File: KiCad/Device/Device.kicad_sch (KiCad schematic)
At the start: 25 parts, among them IC1 ATTINY167-XUR, J1 Mikrofon, J2 Lysføler, J3 Optisk sensor, J4 Fugtføler, J5 VCC, J6 ESP8266(wifi), SW1 Reset, SW2 Button01, SW3 SW_DIP_x01, Y1 Crystal

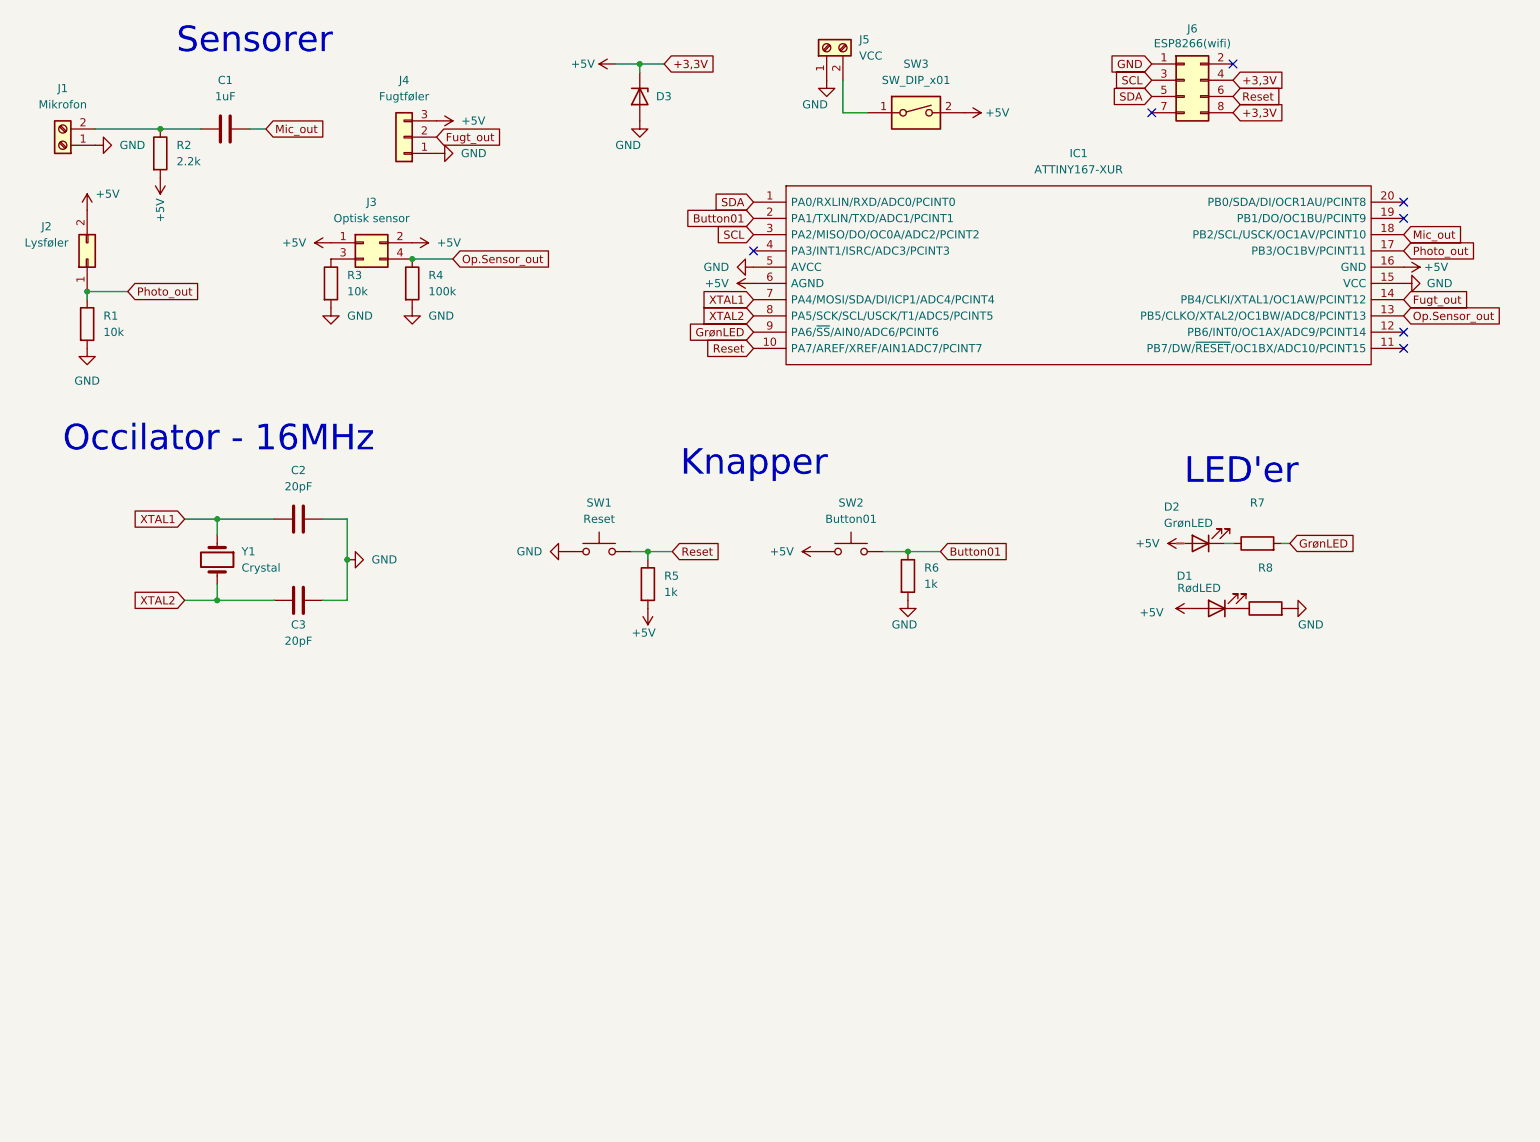
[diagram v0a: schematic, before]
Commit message: Minor fixes
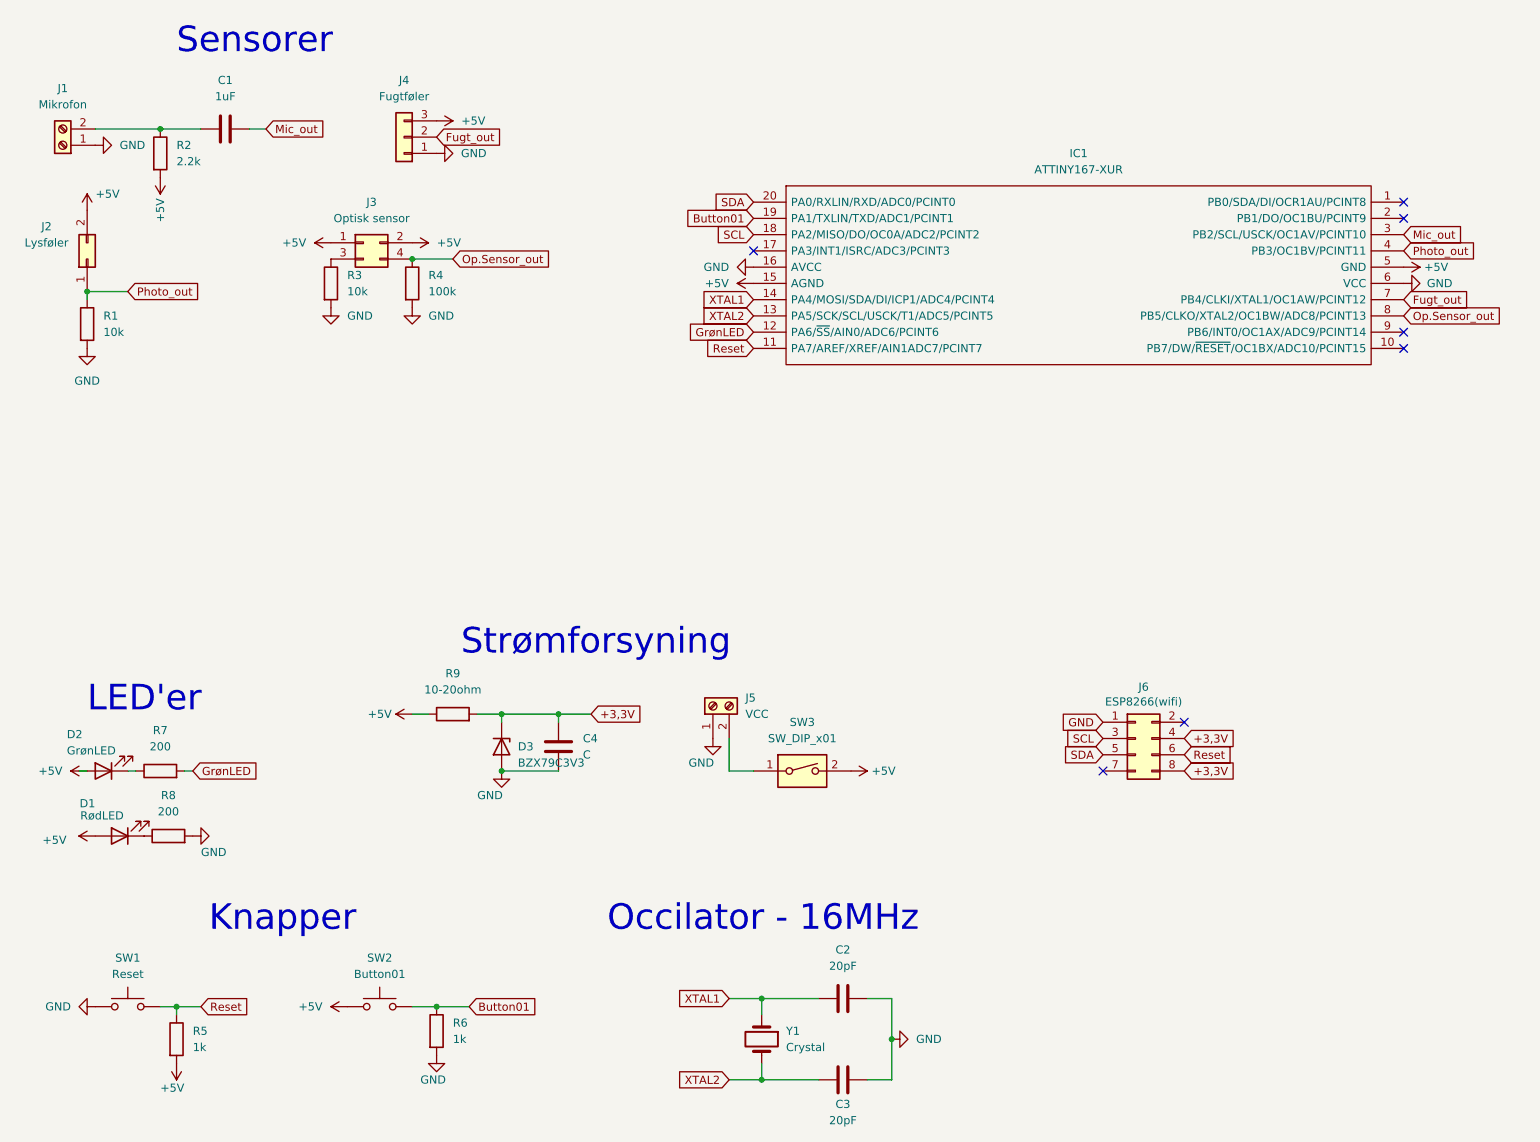
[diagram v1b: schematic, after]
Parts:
- added C4: C, symbol Device:C
- added R9: 10-20ohm, Resistor_THT:R_Axial_DIN0309_L9.0mm_D3.2mm_P12.70mm_Horizontal, symbol Device:R
- D3: value (none) -> BZX79C3V3; footprint (none) -> Diode_SMD:D_MELF_Handsoldering
- IC1: footprint (none) -> Package_DIP:DIP-20_W7.62mm_Socket
- R7, R8: value (none) -> 200
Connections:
- net +5V: now also IC1.15 (AGND), IC1.5 (GND), R9.1; no longer D3.1 (K), IC1.16 (GND), IC1.6 (AGND), J6.4 (Pin_4), J6.8 (Pin_8)
- net Button01: now also IC1.19 (PA1/TXLIN/TXD/ADC1/PCINT1); no longer IC1.2 (PA1/TXLIN/TXD/ADC1/PCINT1)
- net Fugt_out: now also IC1.7 (PB4/CLKI/XTAL1/OC1AW/PCINT12); no longer IC1.14 (PB4/CLKI/XTAL1/OC1AW/PCINT12)
- net GND: now also IC1.16 (AVCC), IC1.6 (VCC), C4.2; no longer IC1.15 (VCC), IC1.5 (AVCC)
- net GrønLED: now also IC1.12 (PA6/~{SS}/AIN0/ADC6/PCINT6); no longer IC1.9 (PA6/~{SS}/AIN0/ADC6/PCINT6)
- net Mic_out: now also IC1.3 (PB2/SCL/USCK/OC1AV/PCINT10); no longer IC1.18 (PB2/SCL/USCK/OC1AV/PCINT10)
- net Op.Sensor_out: now also IC1.8 (PB5/CLKO/XTAL2/OC1BW/ADC8/PCINT13); no longer IC1.13 (PB5/CLKO/XTAL2/OC1BW/ADC8/PCINT13)
- net Photo_out: now also IC1.4 (PB3/OC1BV/PCINT11); no longer IC1.17 (PB3/OC1BV/PCINT11)
- net Reset: now also IC1.11 (PA7/AREF/XREF/AIN1ADC7/PCINT7); no longer IC1.10 (PA7/AREF/XREF/AIN1ADC7/PCINT7)
- net SCL: now also IC1.18 (PA2/MISO/DO/OC0A/ADC2/PCINT2); no longer IC1.3 (PA2/MISO/DO/OC0A/ADC2/PCINT2)
- net SDA: now also IC1.20 (PA0/RXLIN/RXD/ADC0/PCINT0); no longer IC1.1 (PA0/RXLIN/RXD/ADC0/PCINT0)
- net XTAL1: now also IC1.14 (PA4/MOSI/SDA/DI/ICP1/ADC4/PCINT4); no longer IC1.7 (PA4/MOSI/SDA/DI/ICP1/ADC4/PCINT4)
- net XTAL2: now also IC1.13 (PA5/SCK/SCL/USCK/T1/ADC5/PCINT5); no longer IC1.8 (PA5/SCK/SCL/USCK/T1/ADC5/PCINT5)
- new net +3,3V: C4.1, D3.1 (K), J6.4 (Pin_4), J6.8 (Pin_8), R9.2
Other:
- note added: "Strømforsyning"
- moved on the sheet: C2, C3, D1, D2, D3, J5, J6, R5, R6, R7, R8, SW1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

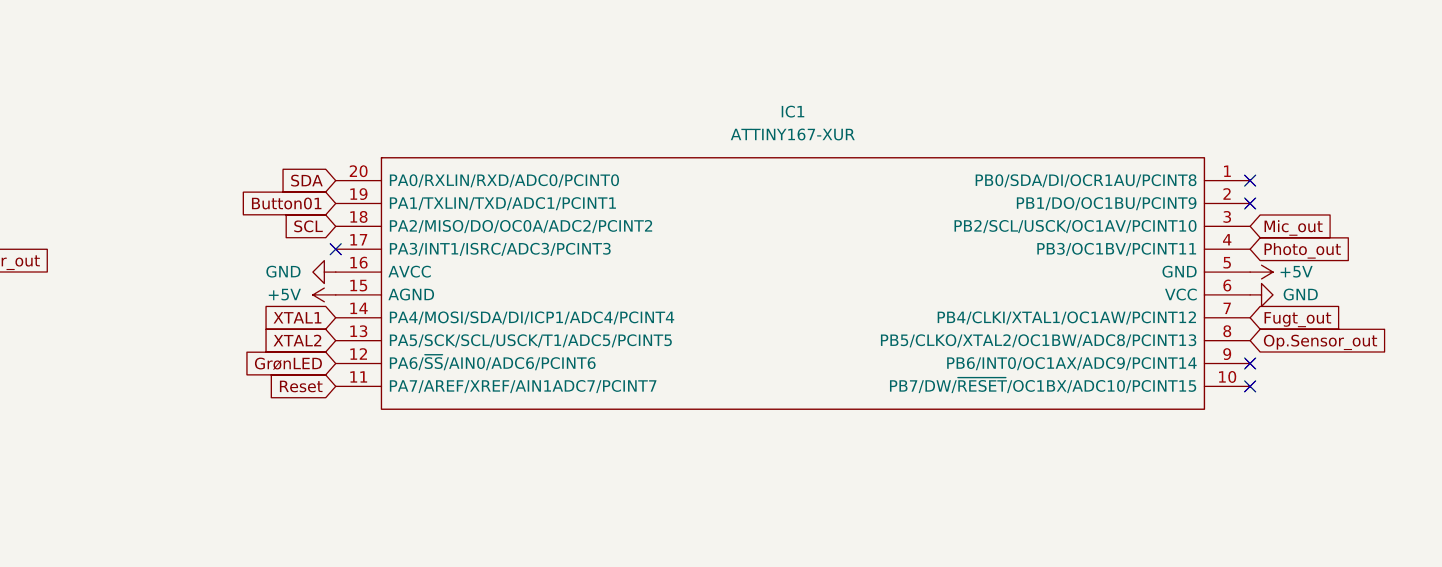
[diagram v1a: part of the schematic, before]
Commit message: fix ic
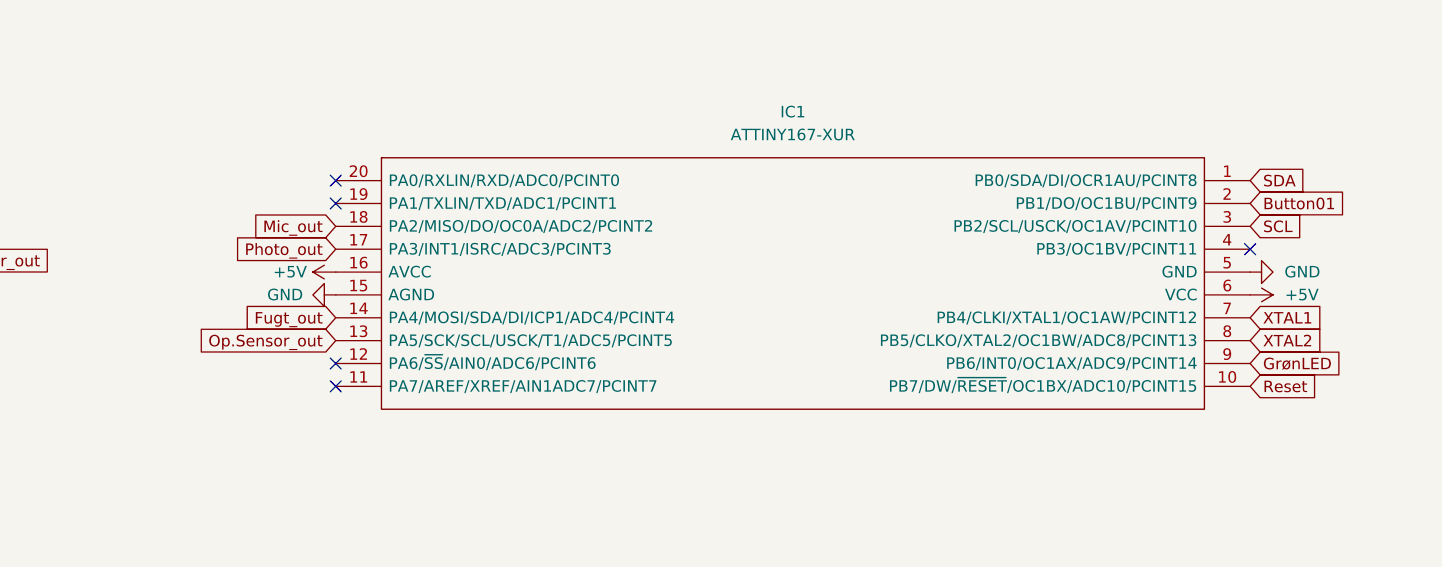
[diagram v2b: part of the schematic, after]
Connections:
- net +5V: now also IC1.16 (AVCC), IC1.6 (VCC); no longer IC1.15 (AGND), IC1.5 (GND)
- net Button01: now also IC1.2 (PB1/DO/OC1BU/PCINT9); no longer IC1.19 (PA1/TXLIN/TXD/ADC1/PCINT1)
- net Fugt_out: now also IC1.14 (PA4/MOSI/SDA/DI/ICP1/ADC4/PCINT4); no longer IC1.7 (PB4/CLKI/XTAL1/OC1AW/PCINT12)
- net GND: now also IC1.15 (AGND), IC1.5 (GND); no longer IC1.16 (AVCC), IC1.6 (VCC)
- net GrønLED: now also IC1.9 (PB6/INT0/OC1AX/ADC9/PCINT14); no longer IC1.12 (PA6/~{SS}/AIN0/ADC6/PCINT6)
- net Mic_out: now also IC1.18 (PA2/MISO/DO/OC0A/ADC2/PCINT2); no longer IC1.3 (PB2/SCL/USCK/OC1AV/PCINT10)
- net Op.Sensor_out: now also IC1.13 (PA5/SCK/SCL/USCK/T1/ADC5/PCINT5); no longer IC1.8 (PB5/CLKO/XTAL2/OC1BW/ADC8/PCINT13)
- net Photo_out: now also IC1.17 (PA3/INT1/ISRC/ADC3/PCINT3); no longer IC1.4 (PB3/OC1BV/PCINT11)
- net Reset: now also IC1.10 (PB7/DW/~{RESET}/OC1BX/ADC10/PCINT15); no longer IC1.11 (PA7/AREF/XREF/AIN1ADC7/PCINT7)
- net SCL: now also IC1.3 (PB2/SCL/USCK/OC1AV/PCINT10); no longer IC1.18 (PA2/MISO/DO/OC0A/ADC2/PCINT2)
- net SDA: now also IC1.1 (PB0/SDA/DI/OCR1AU/PCINT8); no longer IC1.20 (PA0/RXLIN/RXD/ADC0/PCINT0)
- net XTAL1: now also IC1.7 (PB4/CLKI/XTAL1/OC1AW/PCINT12); no longer IC1.14 (PA4/MOSI/SDA/DI/ICP1/ADC4/PCINT4)
- net XTAL2: now also IC1.8 (PB5/CLKO/XTAL2/OC1BW/ADC8/PCINT13); no longer IC1.13 (PA5/SCK/SCL/USCK/T1/ADC5/PCINT5)
